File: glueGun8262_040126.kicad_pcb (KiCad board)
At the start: 2 copper layers, 64 parts, among them CN1 KF243-5.0-2P, CN2 KF243-5.0-2P, CN3 KF243-5.0-2P, CN4 KF243-5.0-2P, CN5 KF243-5.0-2P, CN6 KF243-5.0-2P, CN7 KF243-5.0-2P, CN9 KF243-5.0-4P, U1 DRV8262DDWR, U10 INA240A2DR, U11 INA240A2DR, U2 DRV8262DDWR, U3 ESP32-S3-DEVKITC-1-N8R2, U5 6N137, U6 INA240A2DR, U7 INA240A2DR, U8 K7805-1000R3_C2992391, U9 TLP281-4(GB-TP,J,F

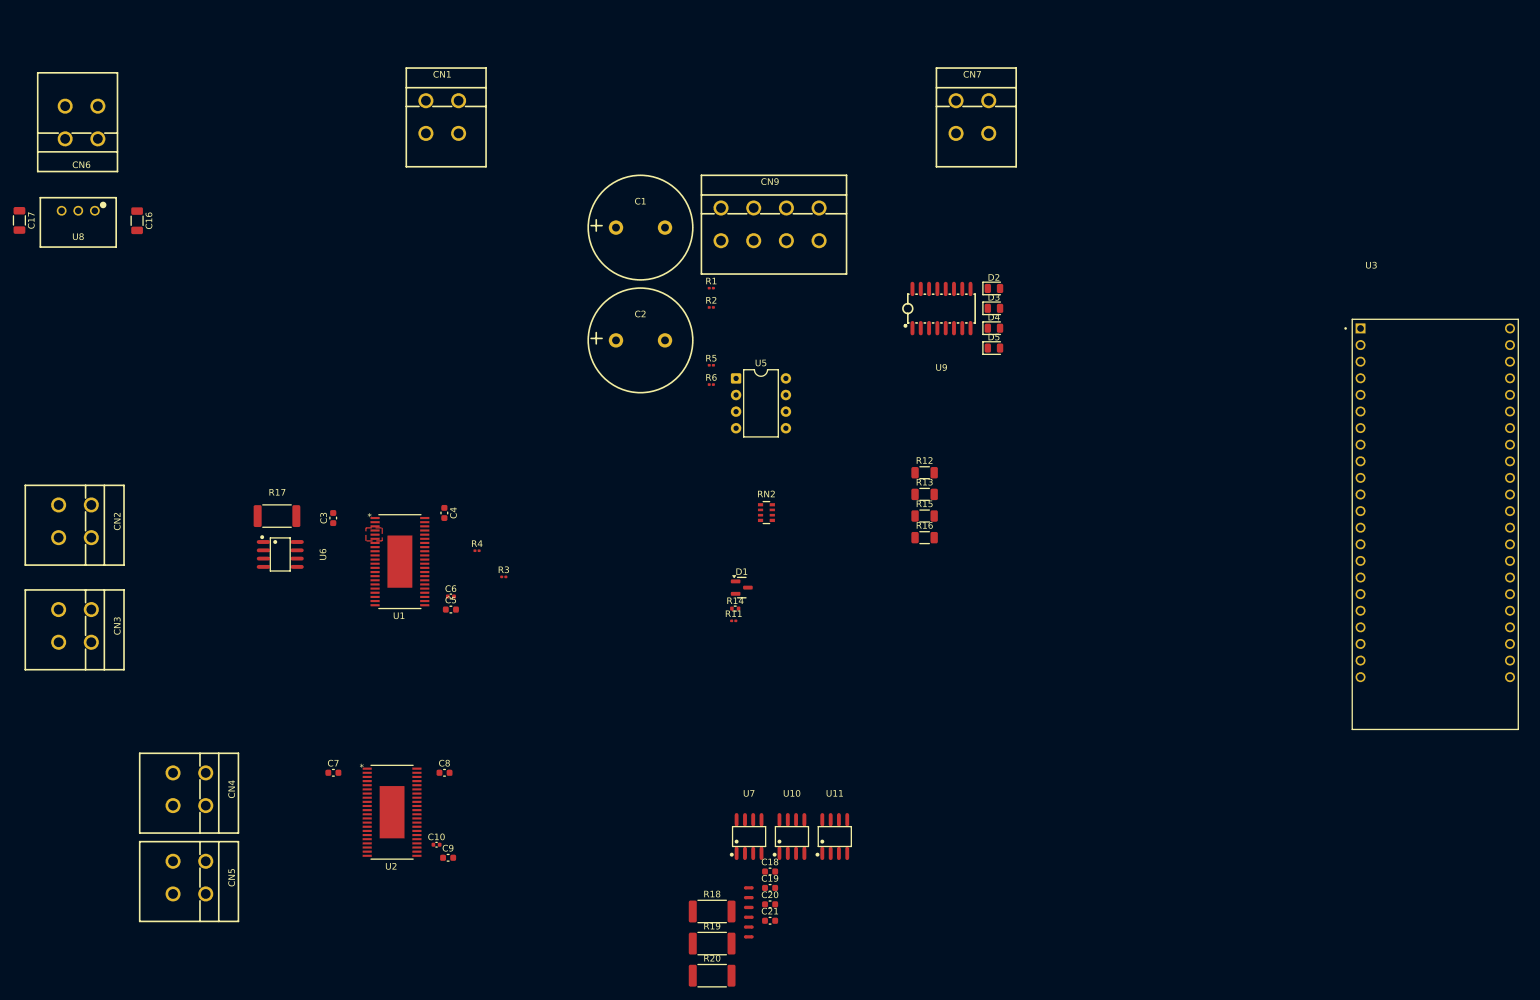
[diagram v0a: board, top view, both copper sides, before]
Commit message: satrted laying pcb
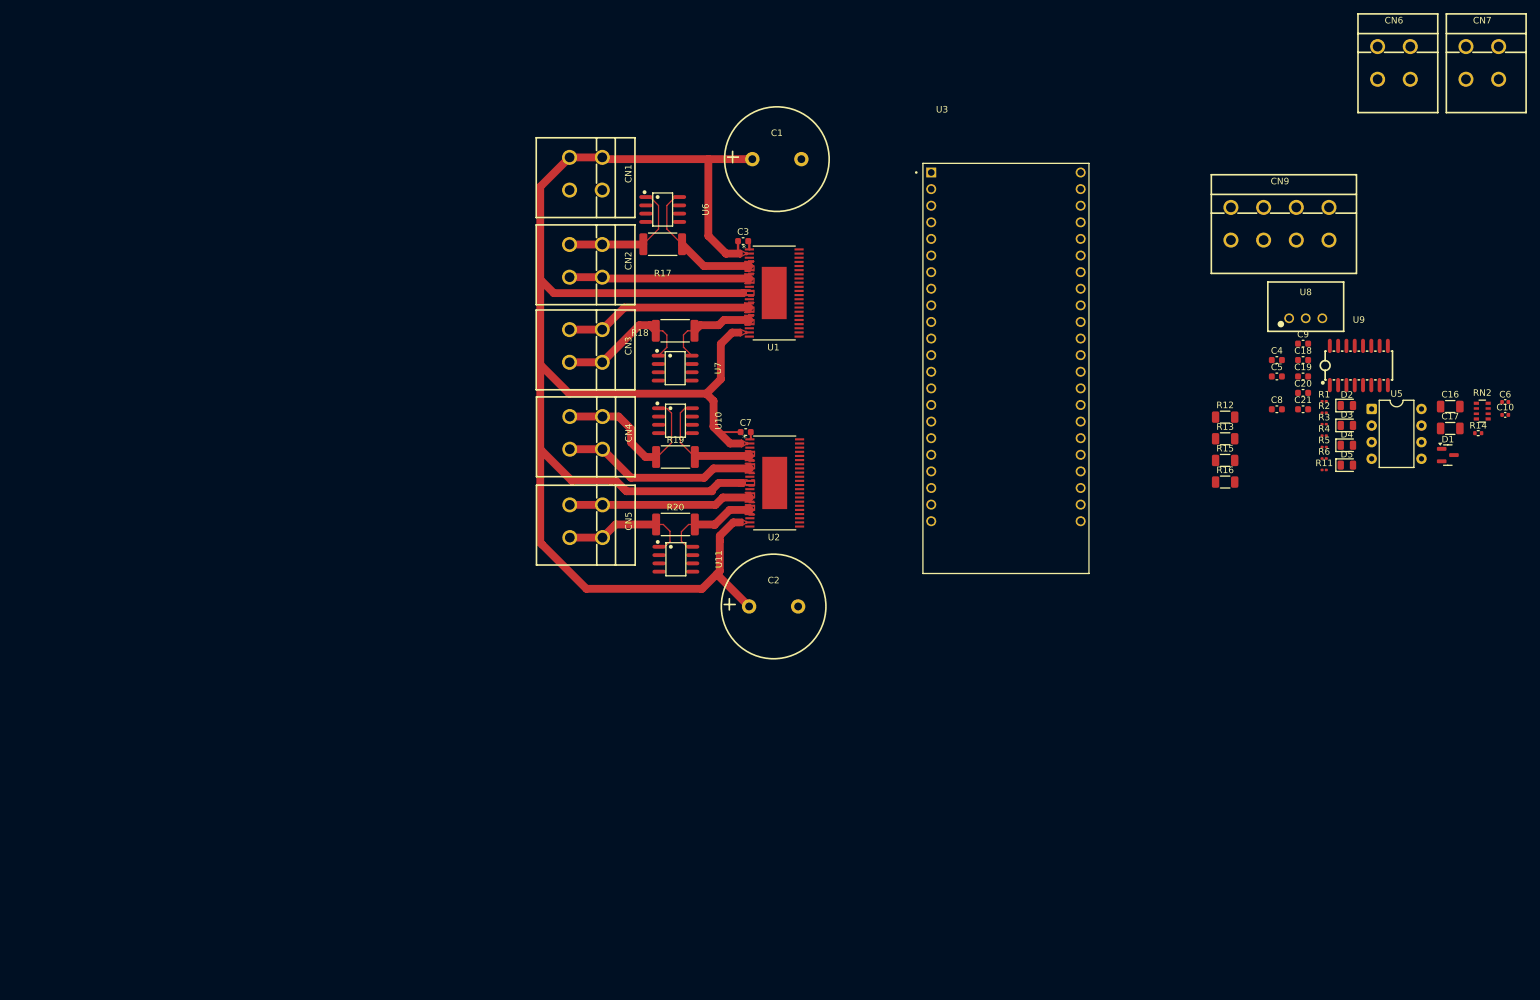
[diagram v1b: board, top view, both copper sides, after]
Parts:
- removed NT1, NT2, NT3, NT4, NT5, NT6, NT7, NT8: NetTie_2, NetTie:NetTie-2_SMD_Pad0.5mm
- moved C17 221.2 mm to (252.9, 99.3), turned to 0 degrees
- moved C16 202.9 mm to (252.9, 95.9), turned to 0 degrees
- moved CN6 201.0 mm to (244.2, 43.4), turned to 0 degrees
- moved U8 188.5 mm to (230.8, 82.4), turned to 0 degrees
- moved C10 176.2 mm to (261.3, 97.2)
- moved C6 164.0 mm to (261.3, 95.3)
- moved C9 152.6 mm to (230.3, 86.3)
- moved C8 138.9 mm to (226.3, 96.4)
- moved C5 131.3 mm to (226.3, 91.3)
- moved R4 130.8 mm to (233.6, 100.4)
- moved C4 129.5 mm to (226.3, 88.8), turned to 0 degrees
- moved R3 127.6 mm to (233.6, 98.6)
- moved R14 116.8 mm to (257.1, 100.0)
- moved C18 113.0 mm to (230.3, 88.8)
- moved C19 113.0 mm to (230.3, 91.3)
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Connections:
- CN2 pad 1: Net-(CN2-Pad1) -> Net-(U6-IN-)
- CN3 pad 2: Net-(CN3-Pad2) -> Net-(U7-IN-)
- CN4 pad 1: Net-(CN4-Pad1) -> Net-(U10-IN-)
- CN5 pad 2: Net-(CN5-Pad2) -> Net-(U11-IN-)
- R17 pad 1: Net-(CN2-Pad1) -> Net-(U6-IN-)
- R18 pad 1: Net-(CN3-Pad2) -> Net-(U7-IN-)
- R19 pad 1: Net-(CN4-Pad1) -> Net-(U10-IN-)
- R20 pad 1: Net-(CN5-Pad2) -> Net-(U11-IN-)
- U10 pad 8: Net-(U10-IN+) -> /U2_OUT1
- U11 pad 8: Net-(U11-IN+) -> /U2_OUT3
- U6 pad 8: Net-(U6-IN+) -> /U1_OUT1
- U7 pad 8: Net-(U7-IN+) -> /U1_OUT3
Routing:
- net +48V: track 0.00 -> 277.0 mm
- net /U2_OUT2: track 0.00 -> 29.9 mm
- net /U1_OUT4: track 0.00 -> 28.9 mm
- net /U2_OUT4: track 0.00 -> 28.0 mm
- net /U1_OUT2: track 0.00 -> 28.0 mm
- net Net-(U10-IN-): track 0.00 -> 26.4 mm
- net Net-(U7-IN-): track 0.00 -> 21.6 mm
- net Net-(U6-IN-): track 0.00 -> 21.4 mm
- net /U1_OUT1: track 0.00 -> 21.0 mm
- net Net-(U11-IN-): track 0.00 -> 20.2 mm
- net /U2_OUT1: track 0.00 -> 18.3 mm
- net /U2_OUT3: track 0.00 -> 15.4 mm
- net /U1_OUT3: track 0.00 -> 14.8 mm
- net Net-(U1-VCP/GND): track 0.00 -> 1.34 mm
- net Net-(U2-VCP/GND): track 0.00 -> 1.17 mm
- added copper zone on F.Cu, net +48V
- added copper zone on F.Cu, net /U1_OUT2
- added copper zone on F.Cu, net /U1_OUT3
- added copper zone on F.Cu, net /U1_OUT4
- added copper zone on F.Cu, net /U2_OUT1
- added copper zone on F.Cu, net /U2_OUT2
- added copper zone on F.Cu, net /U2_OUT3
- added copper zone on F.Cu, net /U2_OUT4
